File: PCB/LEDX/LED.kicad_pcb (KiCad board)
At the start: 2 copper layers, 70 x 70 mm, 26 parts, among them J2 Conn_01x03, J3 TC2030-USB-NL-DS, P1 Square, P2 Square, P3 Square, P4 Square, U1 ICS43434_MEMS_Mic, U2 ESP32-S3-MINI-1, U5 MD8942

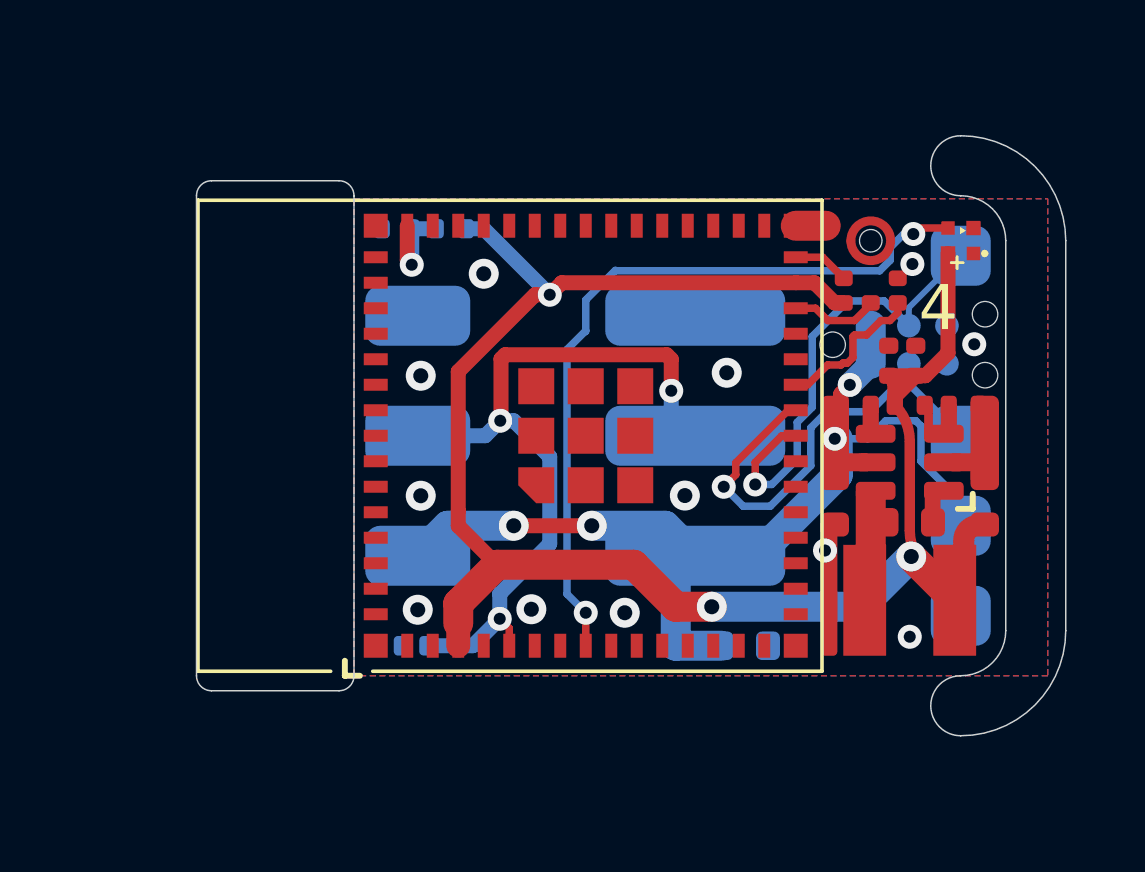
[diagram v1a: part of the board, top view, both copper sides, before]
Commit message: Latest layout
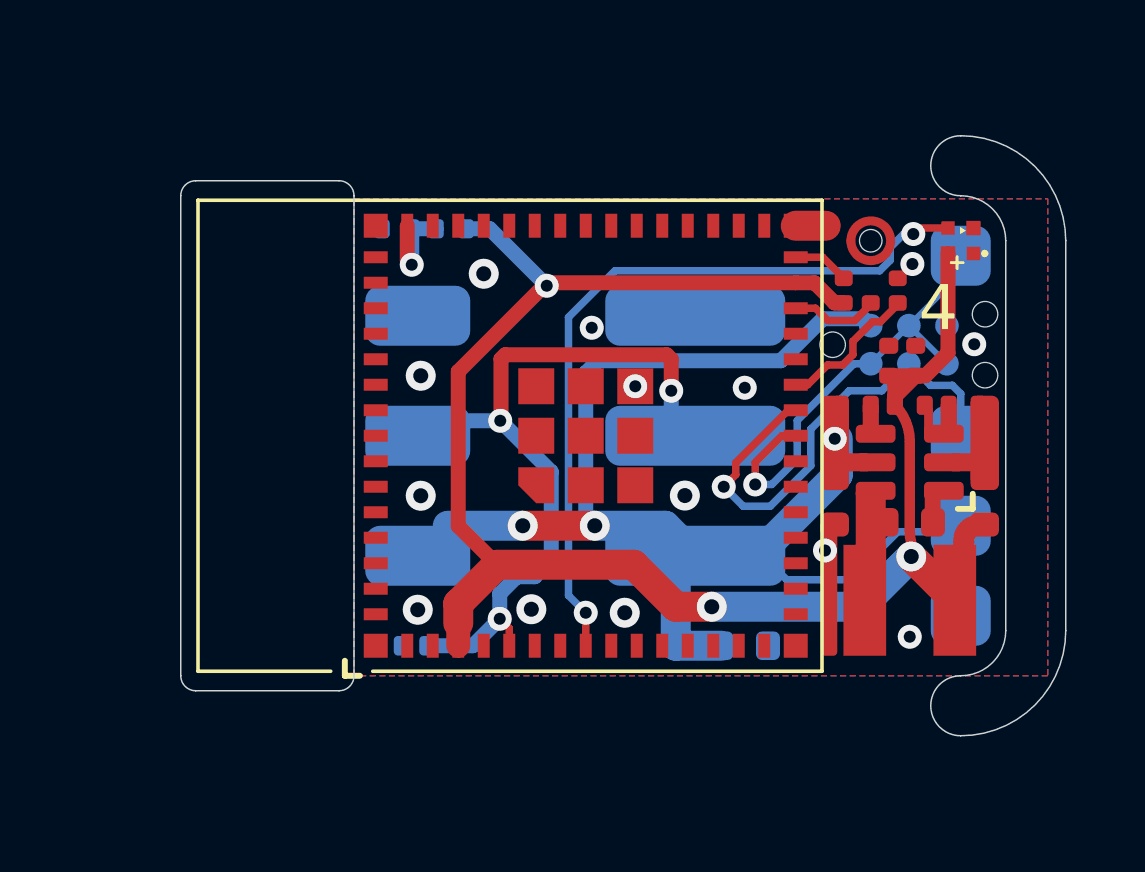
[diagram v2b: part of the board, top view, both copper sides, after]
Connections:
- J3 pad 2: DC -> D-
- J3 pad 6: GND -> D-
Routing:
- net DC: track 32.1 -> 41.4 mm, vias 4 -> 3
- net D-: track 15.6 -> 14.8 mm
- net LED1: track 25.8 -> 25.2 mm
- net GND: vias 12 -> 14
